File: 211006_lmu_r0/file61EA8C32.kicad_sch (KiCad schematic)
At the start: 15 parts, among them U8 ISO7761DBQ

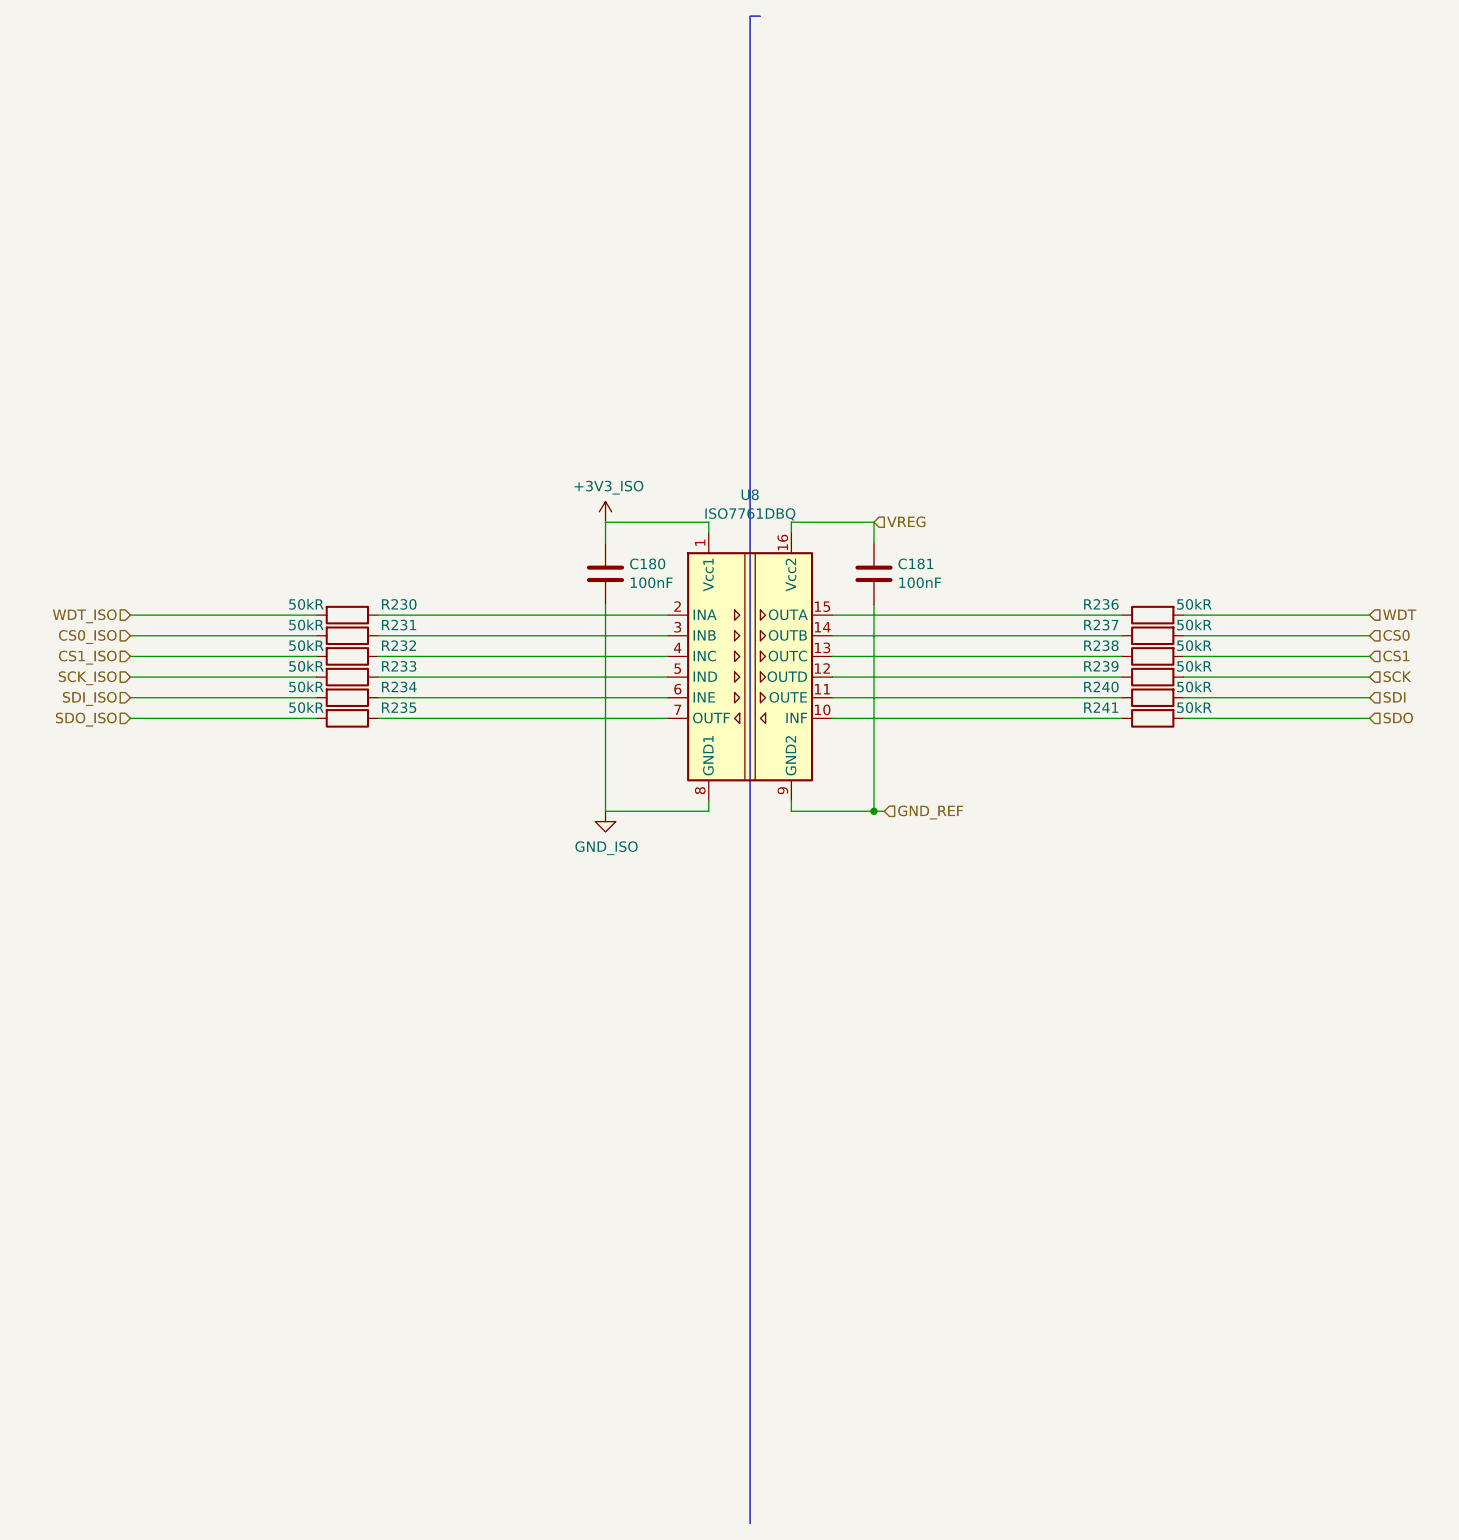
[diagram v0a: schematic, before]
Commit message: merge PCB
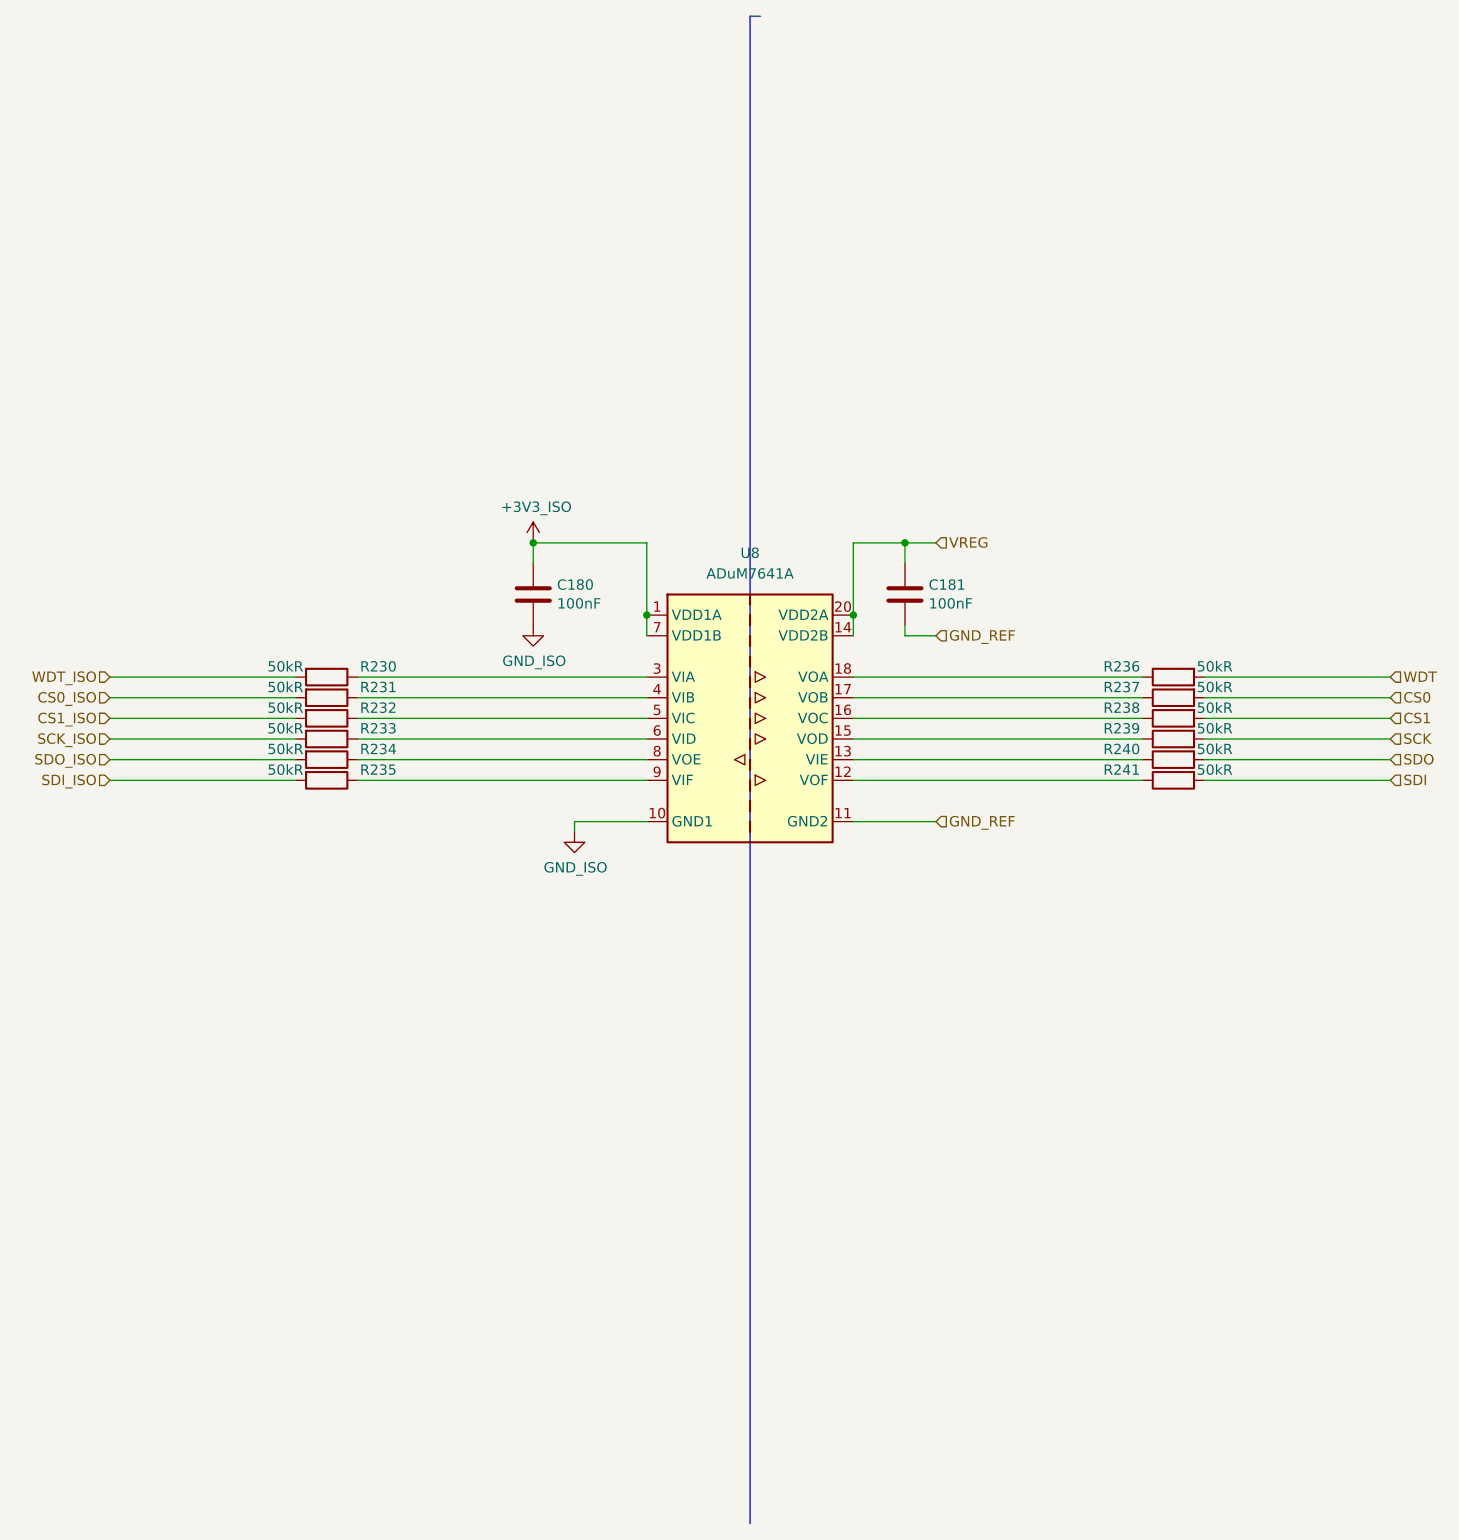
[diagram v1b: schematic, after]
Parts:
- removed U8: ISO7761DBQ, Package_SO:SSOP-16_3.9x4.9mm_P0.635mm, symbol Isolator:ISO7761DBQ
- added U8: ADuM7641A, Package_SO:QSOP-20_3.9x8.7mm_P0.635mm, symbol Isolator:ADuM7641A
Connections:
- net +3V3_ISO: now also U8.1 (VDD1A), U8.7 (VDD1B)
- net GND_ISO: now also U8.10 (GND1), U8.2 (GND1)
- net GND_REF: now also U8.11 (GND2), U8.19 (GND2)
- net SDI: now also R241.2; no longer R240.2
- net SDI_ISO: now also R235.2; no longer R234.2
- net SDO: now also R240.2; no longer R241.2
- net SDO_ISO: now also R234.2; no longer R235.2
- net VREG: now also U8.14 (VDD2B), U8.20 (VDD2A)
- net at R236.1: now also U8.18 (VOA)
- net at R237.1: now also U8.17 (VOB)
- net at R238.1: now also U8.16 (VOC)
- net at R239.1: now also U8.15 (VOD)
- net at R240.1: now also U8.13 (VIE)
- net at R241.1: now also U8.12 (VOF)
- net at R230.1: now also U8.3 (VIA)
- net at R231.1: now also U8.4 (VIB)
- net at R232.1: now also U8.5 (VIC)
- net at R233.1: now also U8.6 (VID)
- net at R234.1: now also U8.8 (VOE)
- net at R235.1: now also U8.9 (VIF)
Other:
- moved on the sheet: C180
